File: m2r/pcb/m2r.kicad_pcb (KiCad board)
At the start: 2 copper layers, 50 x 75 mm, 116 parts, among them IC1 ADP3338, IC10 STM32F303C, IC11 ADP3333, IC2 ADP3335, IC3 ADuM1201, IC4 ADuM1201, IC5 ADuM1201, IC6 MTX2, IC7 ADL5324, IC8 MAX-7Q, IC9 ALM-2712, P1 CONN_2, P2 CONN_2, P3 CONN_4, P4 CONN_4, P5 CONN_4, P6 SWD, P7 SMA, P8 CONN_2, X10 8M, X11 M3 MOUNT, X12 M3 MOUNT, X13 M3 MOUNT, X14 M3 MOUNT

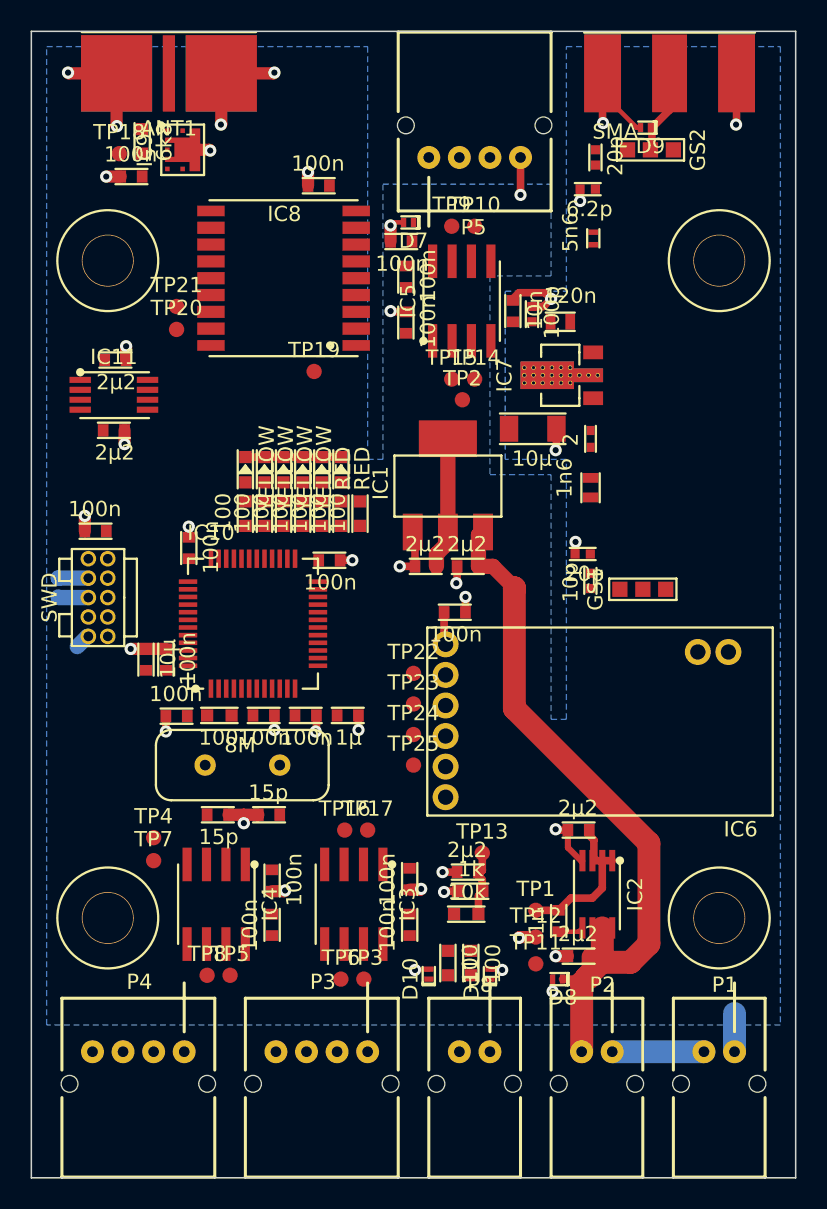
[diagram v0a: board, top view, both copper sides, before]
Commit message: 2 airwires to go
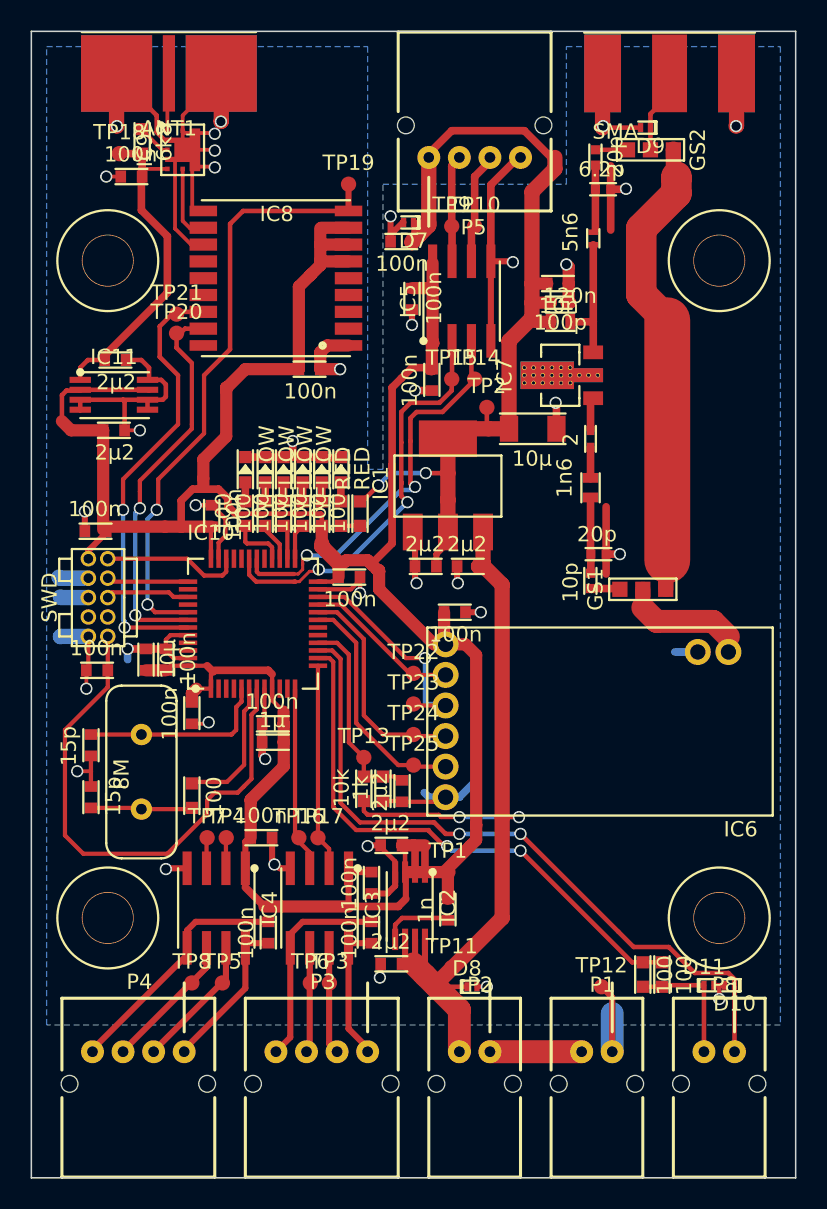
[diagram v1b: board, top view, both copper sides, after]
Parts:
- moved D10 20.0 mm to (162.0, 121.4), turned to 180 degrees
- moved P8 16.0 mm to (162.0, 125.8)
- moved R4 14.0 mm to (157.2, 121.5)
- moved D11 14.0 mm to (160.0, 121.4), turned to 0 degrees
- moved C35 13.4 mm to (119.9, 105.0), turned to 270 degrees
- moved TP19 12.5 mm to (136.8, 69.0)
- moved C8 12.3 mm to (140.2, 112.2)
- moved IC2 12.3 mm to (141.8, 114.0)
- moved C7 12.3 mm to (140.2, 120.0)
- moved C30 12.2 mm to (133.5, 81.1), turned to 0 degrees
- moved R1 11.7 mm to (137.8, 107.8), turned to 270 degrees
- moved R5 11.3 mm to (156.0, 121.5)
- moved TP13 9.96 mm to (137.8, 106.5)
- moved C34 9.95 mm to (121.0, 100.8), turned to 180 degrees
- moved R2 9.92 mm to (139.0, 107.8), turned to 270 degrees
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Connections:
- IC10 pad 14: LED_C -> LED_A
- IC10 pad 15: LED_A -> LED_C
- P8 pad 1: Net-(D11-Pad1) -> LED_C
- P8 pad 2: LED_C -> Net-(D11-Pad1)
- R9 pad 1: Net-(R7-Pad2) -> +5V
- R9 pad 2: +5V -> Net-(R7-Pad2)
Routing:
- net +3.3V: track 12.5 -> 188.9 mm
- net GND: track 84.9 -> 184.1 mm, vias 40 -> 36
- net +5V: track 8.64 -> 65.6 mm, vias 0 -> 2
- net LED_C: track 0.00 -> 46.5 mm, vias 0 -> 2
- net GPS_RESET: track 0.00 -> 40.1 mm, vias 0 -> 2
- net LED_A: track 0.00 -> 36.8 mm, vias 0 -> 2
- net nRST: track 0.00 -> 35.6 mm
- net Net-(GS1-Pad1): track 0.00 -> 31.3 mm
- net GPS_SDA: track 0.00 -> 29.1 mm, vias 0 -> 2
- net RB_TX: track 0.00 -> 27.4 mm, vias 0 -> 2
- net RB_RX: track 0.00 -> 26.7 mm, vias 0 -> 2
- net GPS_SCL: track 0.00 -> 25.8 mm, vias 0 -> 2
- net Net-(C31-Pad1): track 0.00 -> 21.9 mm
- net Net-(C1-Pad1): track 0.00 -> 16.3 mm
- net NTX2B_TXD: track 0.00 -> 15.5 mm, vias 0 -> 1
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
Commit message: 0 airwires!
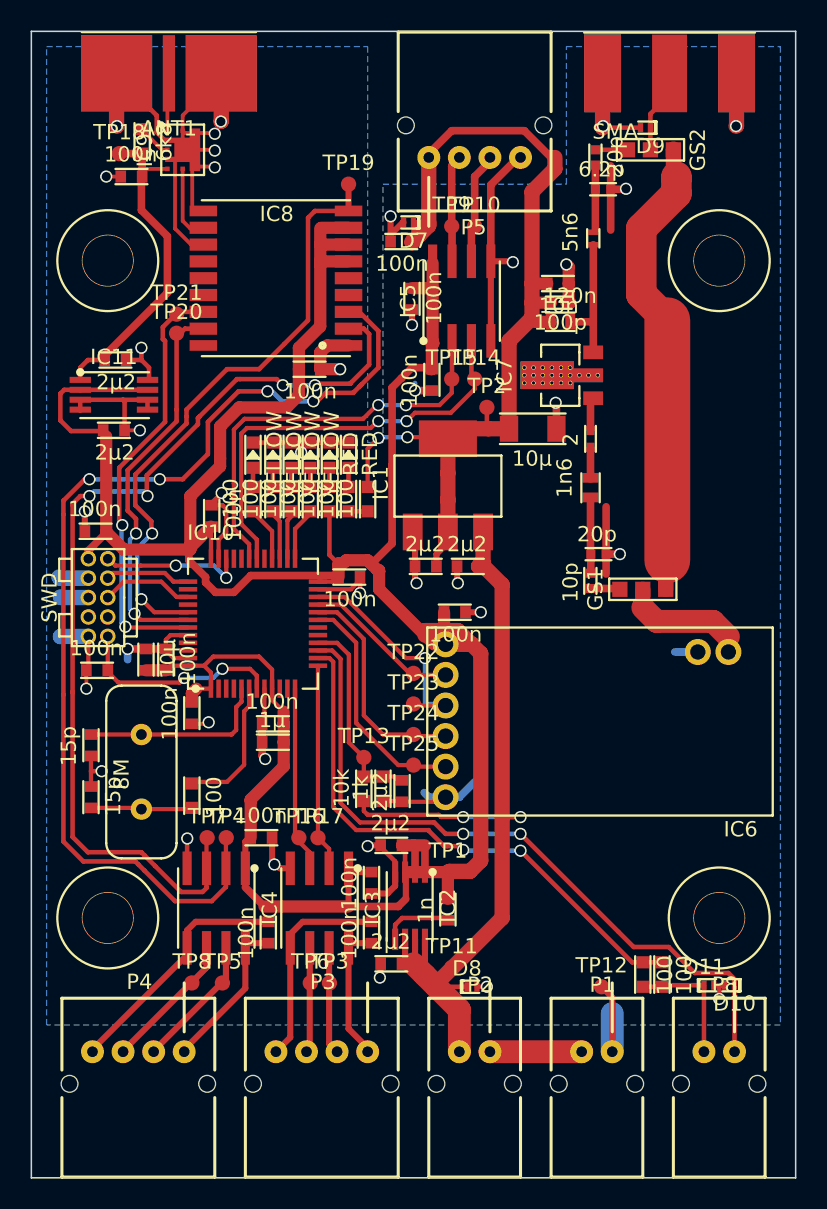
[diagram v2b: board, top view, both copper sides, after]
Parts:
- moved D1 1.07 mm to (135.5, 87.5)
- moved D2 1.07 mm to (136.8, 87.5)
- moved D3 1.07 mm to (134.2, 87.5)
- moved D4 1.07 mm to (131.8, 87.5)
- moved D5 1.07 mm to (133.0, 87.5)
- moved D6 1.07 mm to (130.5, 87.5)
- moved R10 1.07 mm to (134.2, 88.8)
- moved R11 1.07 mm to (131.8, 88.8)
- moved R12 1.07 mm to (133.0, 88.8)
- moved R13 1.07 mm to (130.5, 88.8)
- moved R7 1.07 mm to (136.8, 88.8)
- moved R8 1.07 mm to (135.5, 88.8)
- moved R9 1.07 mm to (138.0, 88.8)
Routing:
- net GPS_RX: track 2.01 -> 69.2 mm, vias 0 -> 4
- net GPS_TX: track 2.02 -> 64.3 mm, vias 0 -> 4
- net nRST: track 35.6 -> 14.0 mm, vias 0 -> 2
- net +3.3V: track 188.9 -> 199.8 mm
- net RB_RX: track 26.7 -> 28.4 mm
- net +5V: track 65.6 -> 67.2 mm
- net GND: track 184.1 -> 182.9 mm, vias 36 -> 37
- net LED_1: track 2.36 -> 3.50 mm
- net LED_2: track 2.25 -> 3.32 mm
- net LED_3: track 2.54 -> 3.29 mm
- net GPS_SDA: track 29.1 -> 28.4 mm
- net SWO: track 5.61 -> 6.11 mm
- net SWDIO: track 9.16 -> 9.57 mm, vias 0 -> 2
